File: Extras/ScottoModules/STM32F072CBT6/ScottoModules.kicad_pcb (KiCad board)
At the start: 2 copper layers, 18 parts, among them J1 USB_C, SW1 SW_Push, U1 STM32F072CBT6, U3 XC6206, U4 USBLC6-2SC6

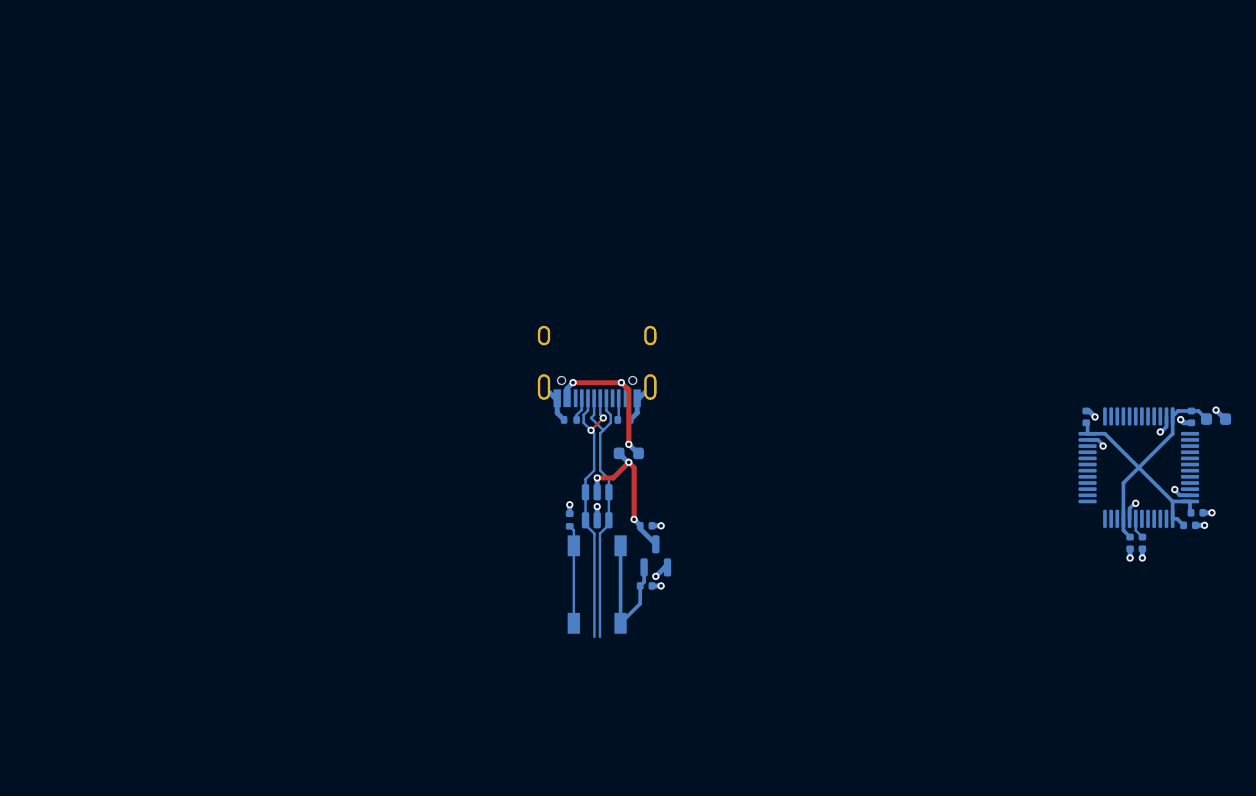
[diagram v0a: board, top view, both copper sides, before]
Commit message: Modified PCB Project
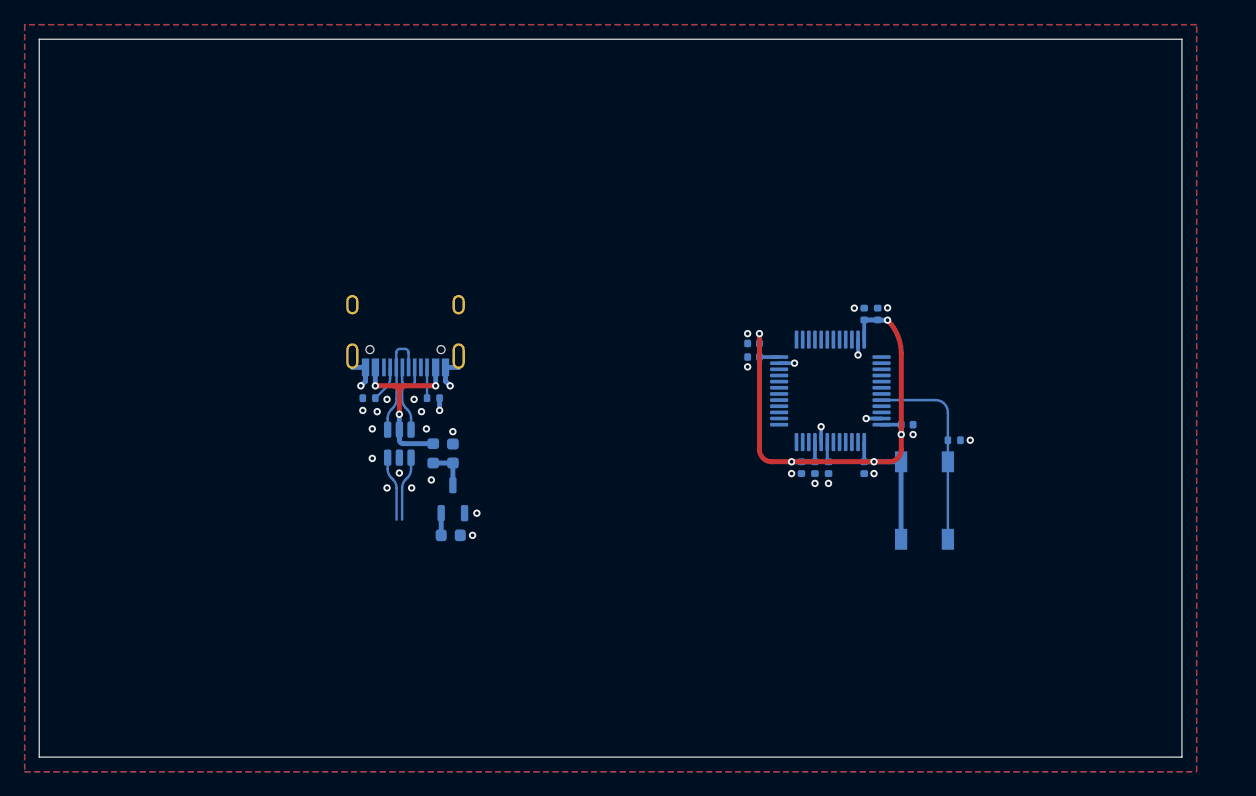
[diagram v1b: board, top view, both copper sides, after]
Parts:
- removed U4: USBLC6-2SC6, ScottoKeebs_Components:ESD_SOT-23-6
- added C10: 100nF, Capacitor_SMD:C_0402_1005Metric, B.Cu at (155.9, 87.8)
- added C11: 4.7uF, Capacitor_SMD:C_0402_1005Metric, B.Cu at (157.0, 87.8)
- added U2: USBLC6-2SC6, Package_TO_SOT_SMD:SOT-23-6, B.Cu at (118.1, 98.4)
- C1, C4, C5, C7, C9: footprint ScottoKeebs_Components:Capacitor_0402 -> Capacitor_SMD:C_0402_1005Metric
- C2, C3: value 100nF -> 1uF; footprint ScottoKeebs_Components:Capacitor_0402 -> Capacitor_SMD:C_0603_1608Metric
- C6: value 10uF -> 4.7uF; footprint ScottoKeebs_Components:Capacitor_0603 -> Capacitor_SMD:C_0402_1005Metric
- C8: value 1uF -> 10nF; footprint ScottoKeebs_Components:Capacitor_0402 -> Capacitor_SMD:C_0402_1005Metric
- F1: footprint ScottoKeebs_Components:Fuse_0603 -> Fuse:Fuse_0603_1608Metric
- J1: value USB_C -> USB_C_Receptacle_USB2.0_16P; footprint ScottoKeebs_Components:USB_C_HRO_TYPE-C-31-M-12 -> Connector_USB:USB_C_Receptacle_HRO_TYPE-C-31-M-12
- R1: value 10k -> 5.1k; footprint ScottoKeebs_Components:Resistor_0402 -> Resistor_SMD:R_0402_1005Metric
- R2: footprint ScottoKeebs_Components:Resistor_0402 -> Resistor_SMD:R_0402_1005Metric
- R3: value 5.1k -> 10k; footprint ScottoKeebs_Components:Resistor_0402 -> Resistor_SMD:R_0402_1005Metric
- SW1: footprint ScottoKeebs_Components:Button_TL3342 -> Button_Switch_SMD:SW_SPST_TL3342
- U1: footprint ScottoKeebs_Components:Package_LQFP-48_7x7mm_P0.5 -> Package_QFP:LQFP-48_7x7mm_P0.5mm
- U3: value XC6206 -> XC6206PxxxMR; footprint ScottoKeebs_Components:Voltage_SOT-23 -> Package_TO_SOT_SMD:SOT-23-3
- moved C2 55.5 mm to (122.4, 99.2), turned to -90 degrees
- moved C3 52.5 mm to (122.3, 105.8), turned to 180 degrees
- moved C5 38.2 mm to (146.9, 91.3), turned to 0 degrees
- moved C6 38.1 mm to (146.9, 90.2), turned to 0 degrees
- moved C1 29.7 mm to (153.0, 100.3), turned to -90 degrees
- moved SW1 27.5 mm to (160.8, 103.0), turned to -90 degrees
- moved C4 26.9 mm to (155.9, 100.3)
- moved R3 26.9 mm to (163.2, 98.1), turned to 180 degrees
- moved U1 25.8 mm to (153.1, 94.1)
- moved C7 21.4 mm to (159.4, 96.8), turned to 180 degrees
- moved R1 19.1 mm to (115.6, 94.7), turned to 180 degrees
- moved U3 17.1 mm to (122.4, 102.9)
- moved F1 15.9 mm to (120.8, 99.2), turned to -90 degrees
- moved C9 15.9 mm to (150.8, 100.3), turned to 90 degrees
- moved J1 15.8 mm to (118.6, 88.1)
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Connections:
- net A0 renamed /A0
- net A1 renamed /A1
- net A10 renamed /A10
- net A13 renamed /A13
- net A14 renamed /A14
- net A15 renamed /A15
- net A2 renamed /A2
- net A3 renamed /A3
- net A4 renamed /A4
- net A5 renamed /A5
- net A6 renamed /A6
- net A7 renamed /A7
- net A8 renamed /A8
- net A9 renamed /A9
- net B0 renamed /B0
- net B1 renamed /B1
- net B10 renamed /B10
- net B11 renamed /B11
- net B12 renamed /B12
- net B13 renamed /B13
- net B14 renamed /B14
- net B15 renamed /B15
- net B2 renamed /B2
- net B3 renamed /B3
- net B4 renamed /B4
- net B5 renamed /B5
- net B6 renamed /B6
- net B7 renamed /B7
- net B8 renamed /B8
- net B9 renamed /B9
- net C13 renamed /C13
- net C14 renamed /C14
- net C15 renamed /C15
- net F0 renamed /F0
- net F1 renamed /F1
- C1 pad 1: GND -> /NRST
- C1 pad 2: +3.3V -> GND
- C2 pad 2: +3.3V -> +5V
- C7 pad 1: Net-(U1-NRST) -> GND
- C7 pad 2: GND -> +3.3V
- C8 pad 1: +5V -> GND
- C8 pad 2: GND -> +3.3V
- C9 pad 1: +3.3V -> GND
- C9 pad 2: GND -> +3.3V
- J1 pad A6: D+ -> /USB-D+
- J1 pad A7: D- -> /USB-D-
- J1 pad A8: (no net) -> unconnected-(J1-SBU1-PadA8)
- J1 pad B6: D+ -> /USB-D+
- J1 pad B7: D- -> /USB-D-
- J1 pad B8: (no net) -> unconnected-(J1-SBU2-PadB8)
- R1 pad 1: GND -> Net-(J1-CC1)
- R1 pad 2: BOOT0 -> GND
- R2 pad 1: Net-(J1-CC1) -> Net-(J1-CC2)
- R3 pad 1: Net-(J1-CC2) -> GND
- R3 pad 2: GND -> /BOOT0
- SW1 pad 2: BOOT0 -> /BOOT0
- U1 pad 32: D- -> /MCU-D-
- U1 pad 33: D+ -> /MCU-D+
- U1 pad 44: BOOT0 -> /BOOT0
- U1 pad 7: Net-(U1-NRST) -> /NRST
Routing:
- net D-: track 23.7 -> 0.00 mm, vias 2 -> 0
- net D+: track 23.6 -> 0.00 mm
- net /BOOT0: track 0.00 -> 16.2 mm
- net +3.3V: track 42.7 -> 58.4 mm, vias 0 -> 5
- net GND: track 23.8 -> 13.3 mm, vias 16 -> 32
- net +5V: track 12.9 -> 3.40 mm, vias 3 -> 0
- net /USB-D-: track 0.00 -> 8.99 mm
- net BOOT0: track 8.55 -> 0.00 mm
- net /USB-D+: track 0.00 -> 8.26 mm
- net /MCU-D-: track 0.00 -> 5.24 mm
- net /MCU-D+: track 0.00 -> 5.24 mm
- net VBUS: track 13.2 -> 16.2 mm
- net Net-(U1-NRST): track 1.70 -> 0.00 mm
- net /NRST: track 0.00 -> 1.60 mm
- net Net-(J1-CC1): track 1.93 -> 2.95 mm
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- added copper zone on B.Cu, net GND
- added copper zone on F.Cu, net GND
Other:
- board outline added: 92.9 x 58.3 mm
- board text added: "Bootloader"
- board text removed: "JLCJLCJLCJLC"
